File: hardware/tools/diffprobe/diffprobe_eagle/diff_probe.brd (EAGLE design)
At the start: 26.7 x 26.3 mm, 32 parts, among them U1 AD8129, X1 SMA-142-0701-801/806

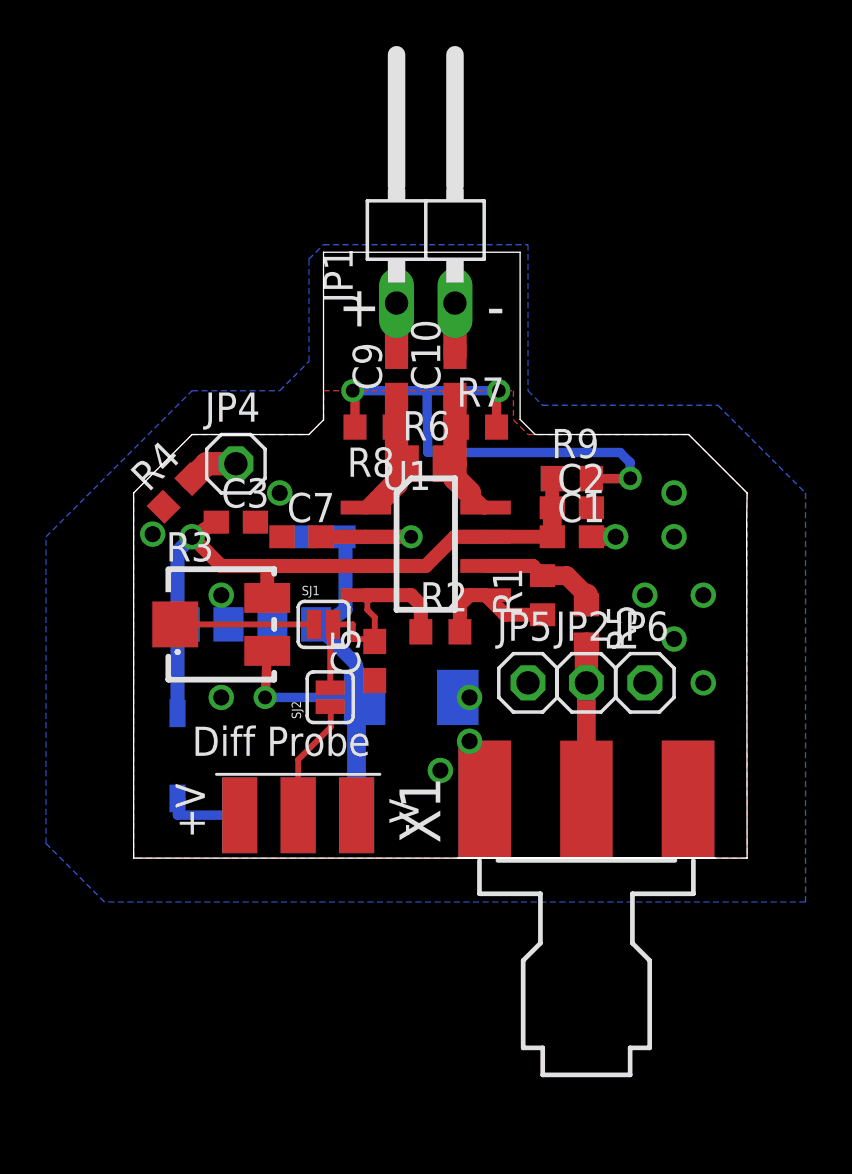
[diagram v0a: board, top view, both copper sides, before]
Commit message: HW: Update differential probe with latest design
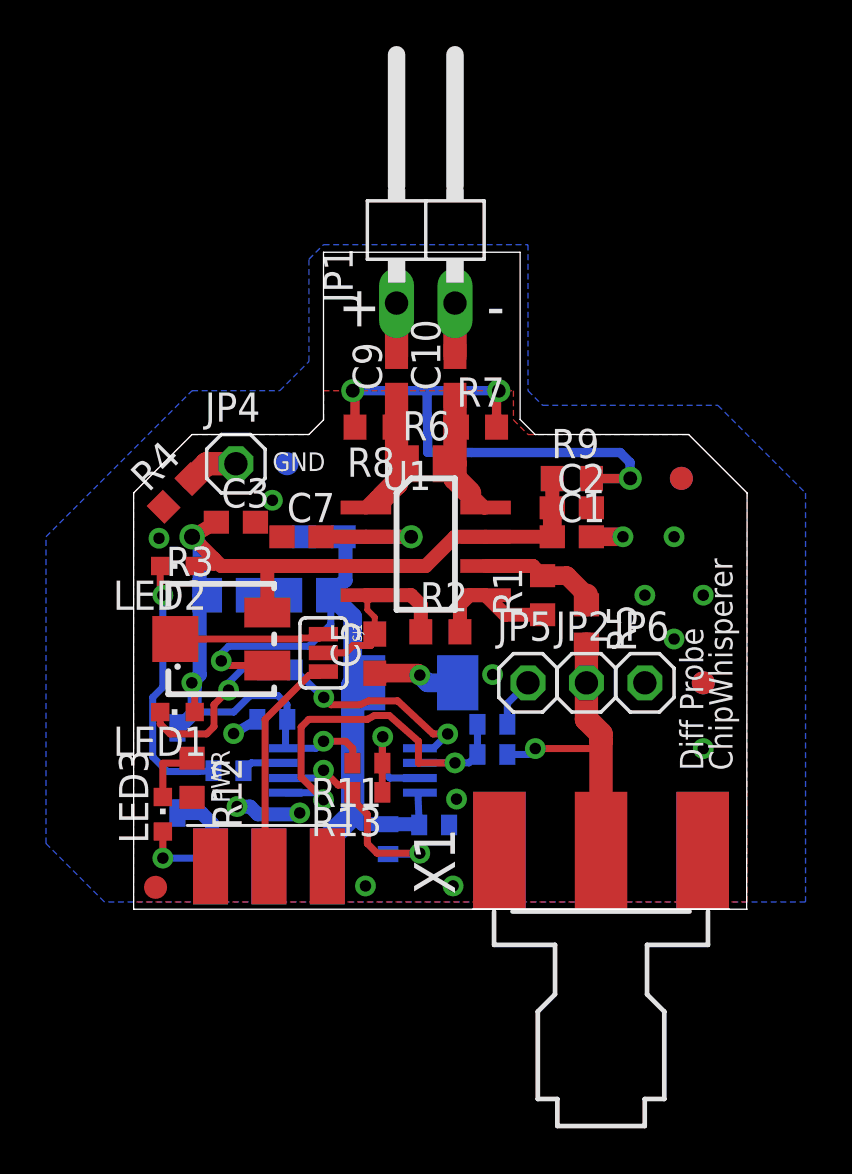
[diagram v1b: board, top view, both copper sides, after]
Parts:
- removed SJ2: SOLDERJUMPERNC, SparkFun:SJ_2S
- added C11, C12, C13: (no value), resistor:C0402
- added LED1, LED3: RIGHT, led:CHIPLED_0603
- added LED2: LEFT, led:CHIPLED_0603
- added R11, R14: 10k, 1%, rcl:R0402
- added R12: 4k7, resistor:R0603
- added R13: 510R, 1%, rcl:R0402
- added R15: 25k, rcl:R0402
- added R16, R17: (no value), rcl:R0402
- added U$1, U$2, U$3, U$4, U$5, U$6: FIDUCIAL, adafruit:FIDUCIAL_1MM
- added U2: LM2903PWR, Texas Instruments_By_element14_Batch_1:SOP65P640X120-8N
- SJ1: value SOLDERJUMPERNC -> (none); device SparkFun:SJ_2S -> SparkFun:SJ_3_PASTE1&2
- moved JP3 2.56 mm to (17.3, 13.0)
- moved X1 2.31 mm to (31.8, 11.1)
- moved C6 1.60 mm to (15.6, 24.8)
- moved C8 1.42 mm to (19.1, 24.8)
- moved SJ1 1.24 mm to (19.7, 22.3), turned to 270 degrees
- moved D1 0.64 mm to (13.3, 17.1)
- moved R3 0.64 mm to (15.2, 22.9)
- moved D2 0.63 mm to (23.5, 21.0)
- moved C5 0.32 mm to (21.9, 22.2)
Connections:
- new net N$16: R11.1, R13.1, U2.3
- new net N$17: R13.2, R14.1, U2.6
- new net N$18: R16.1, U2.1
- new net N$19: C11.2, R15.2, U2.2, U2.5
- new net N$20: LED1.C, R16.2
- new net N$21: R17.1, U2.7
- new net N$22: LED2.C, R17.2
- new net N$9: LED3.C, R12.1
- net AGND: now also C11.1, C12.2, C13.1, R12.2
- net N$1: now also LED3.A
- net N$10: now also SJ1.3; no longer SJ2.1
- net N$12: now also R15.1
- net N$2: now also C12.1, LED1.A, LED2.A, R11.2, U2.8
- net N$3: no longer SJ2.2
- net N$8: now also C13.2, R14.2, U2.4
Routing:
- net N$19: track 0.00 -> 17.6 mm, vias 0 -> 2
- net N$2: track 30.2 -> 45.5 mm, vias 1 -> 3
- net N$22: track 0.00 -> 11.4 mm, vias 0 -> 1
- net N$17: track 0.00 -> 10.6 mm, vias 0 -> 2
- net AGND: track 1.05 -> 11.4 mm, vias 14 -> 16
- net N$8: track 27.2 -> 37.3 mm
- net N$18: track 0.00 -> 9.34 mm, vias 0 -> 2
- net N$20: track 0.00 -> 7.24 mm, vias 0 -> 1
- net N$12: track 6.74 -> 13.5 mm, vias 0 -> 1
- net N$16: track 0.00 -> 6.16 mm, vias 0 -> 1
- net N$10: track 5.32 -> 10.5 mm
- net N$1: track 3.52 -> 6.94 mm, vias 0 -> 1
- net N$9: track 0.00 -> 2.83 mm
- net N$3: track 11.2 -> 8.54 mm
- net N$21: track 0.00 -> 1.97 mm
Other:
- board size 26.7 x 26.3 mm -> 26.7 x 28.6 mm
- board text added: "28OCT2014"
- board text added: "ChipWhisperer"
- board text added: "GND"
- board text added: "NPCB-DIFFPROBE-02"
- board text added: "NewAE Technology Inc"
- board text added: "PWR"
- board text added: "V+"
- board text added: "V-"
- board text removed: "+V"
- board text removed: "-V"
- board text removed: "ChipWhisperer.com"
- board text removed: "Colin O'Flynn"
- board text removed: "MAR92013"

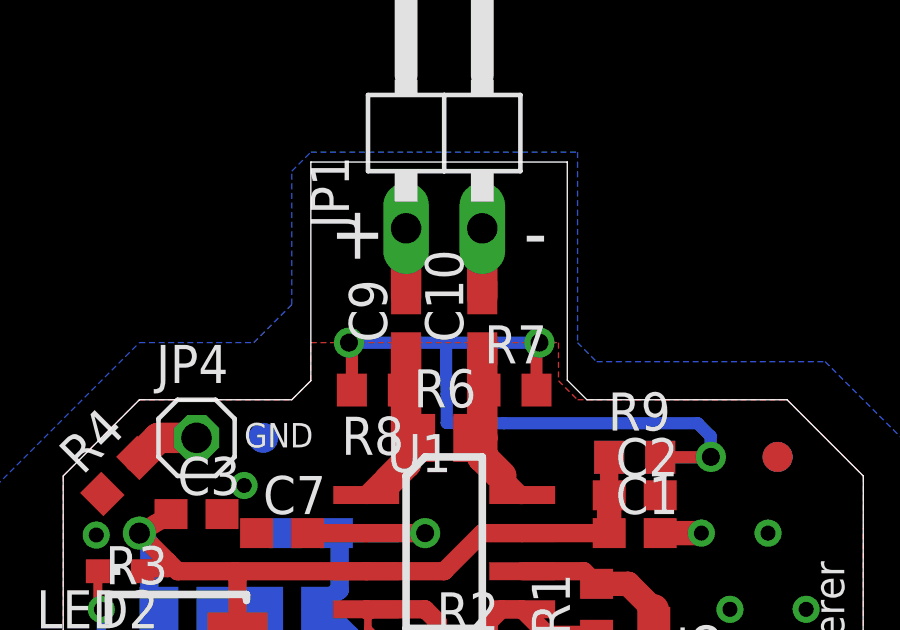
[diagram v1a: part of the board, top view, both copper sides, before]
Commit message: Update differential probe stuff
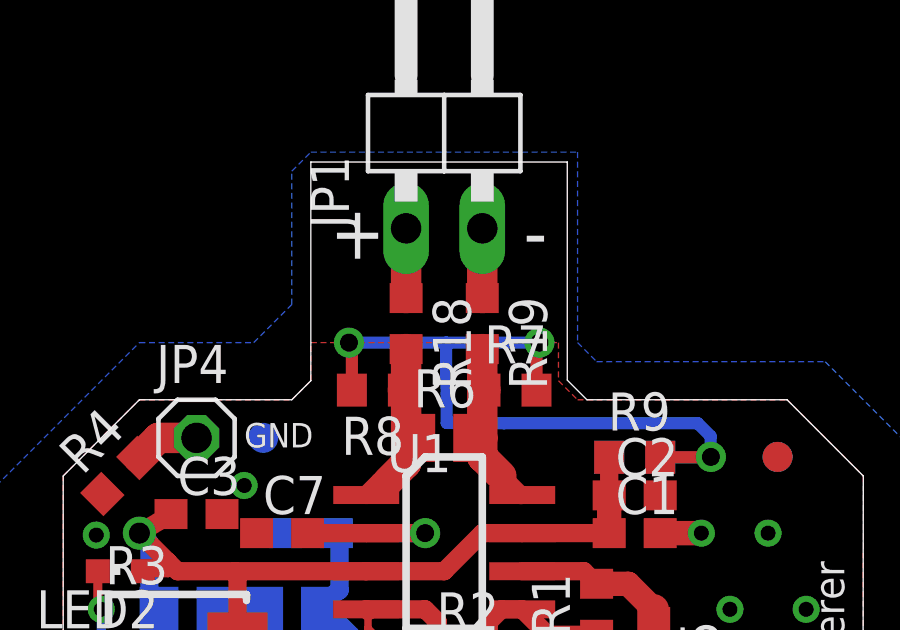
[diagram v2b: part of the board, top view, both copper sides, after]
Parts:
- removed C10, C9: 0R, rcl:C0603
- added R18, R19: 10R, resistor:R0603
- C11: value (none) -> 680pF
- C12, C13: value (none) -> 100nF
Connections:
- net N$13: now also R19.2; no longer C10.1
- net N$14: now also R19.1; no longer C10.2
- net N$6: now also R18.1; no longer C9.2
- net N$7: now also R18.2; no longer C9.1
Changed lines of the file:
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@@
 <element name="JP6" library="pinhead" package="1X01" value="" x="33.655" y="20.955"/>
 <element name="R5" library="resistor" package="R0603" value="49.9R" x="31.115" y="23.495" rot="R270"/>
-<element name="C9" library="rcl" package="C0603" value="0R" x="22.86" y="34.300159375" rot="R90"/>
-<element name="C10" library="rcl" package="C0603" value="0R" x="25.4" y="34.3001625" rot="R90"/>
 <element name="R6" library="resistor" package="M0805" value="DNM" x="24.13" y="30.48"/>
 <element name="R7" library="resistor" package="R0603" value="DNM" x="26.35758125" y="32.072578125"/>
@@
 <element name="R14" library="rcl" package="R0402" value="10k, 1%" x="22.491703125" y="14.160503125" rot="MR90"/>
 <element name="R15" library="rcl" package="R0402" value="25k" x="27.0256" y="17.840959375" rot="MR0"/>
-<element name="C11" library="resistor" package="C0402" value="" x="27.025603125" y="19.1516" rot="MR0">
+<element name="C11" library="resistor" package="C0402" value="680pF" x="27.025603125" y="19.1516" rot="MR0">
 <attribute name="SPICEPREFIX" value="C" x="27.025603125" y="19.1516" size="1.778" layer="28" rot="MR0" display="off"/>
 </element>
@@
 <element name="LED1" library="led" package="CHIPLED_0603" value="RIGHT" x="13.335" y="19.685" rot="R90"/>
 <element name="LED2" library="led" package="CHIPLED_0603" value="LEFT" x="13.335" y="26.035" rot="R90"/>
-<element name="C12" library="resistor" package="C0402" value="" x="17.457421875" y="19.3675" rot="MR0">
+<element name="C12" library="resistor" package="C0402" value="100nF" x="17.457421875" y="19.3675" rot="MR0">
 <attribute name="SPICEPREFIX" value="C" x="17.457421875" y="19.3675" size="1.778" layer="28" rot="MR0" display="off"/>
 </element>
-<element name="C13" library="resistor" package="C0402" value="" x="24.492421875" y="14.77758125" rot="MR0">
+<element name="C13" library="resistor" package="C0402" value="100nF" x="24.492421875" y="14.77758125" rot="MR0">
 <attribute name="SPICEPREFIX" value="C" x="24.492421875" y="14.77758125" size="1.778" layer="28" rot="MR0" display="off"/>
 </element>
@@
 <element name="U$5" library="adafruit" package="FIDUCIAL_1MM" value="FIDUCIAL" x="36.195" y="20.955"/>
 <element name="U$6" library="adafruit" package="FIDUCIAL_1MM" value="FIDUCIAL" x="36.195" y="20.955" rot="MR0"/>
+<element name="R18" library="resistor" package="R0603" value="10R" x="22.86" y="34.29" rot="R270"/>
+<element name="R19" library="resistor" package="R0603" value="10R" x="25.4" y="34.29" rot="R270"/>
 </elements>
 <signals>
@@
 <signal name="N$6">
 <contactref element="JP1" pad="1"/>
-<contactref element="C9" pad="2"/>
-<wire x1="22.86" y1="35.150159375" x2="22.86" y2="37.465" width="1.016" layer="1"/>
+<contactref element="R18" pad="1"/>
+<wire x1="22.86" y1="35.14" x2="22.86" y2="37.465" width="1.016" layer="1"/>
 </signal>
 <signal name="N$7">
-<contactref element="C9" pad="1"/>
 <contactref element="R6" pad="1"/>
 <contactref element="R8" pad="1"/>
 <contactref element="U1" pad="1"/>
-<wire x1="22.86" y1="33.450159375" x2="22.86" y2="31.75" width="1.016" layer="1"/>
 <wire x1="22.86" y1="31.75" x2="22.86" y2="30.48" width="1.016" layer="1"/>
 <wire x1="22.86" y1="30.48" x2="22.86" y2="29.63418125" width="1.016" layer="1"/>
@@
 <wire x1="22.25801875" y1="29.0322" x2="21.9872" y2="29.0322" width="0.6096" layer="1"/>
 <wire x1="21.9872" y1="29.0322" x2="21.53" y2="28.575" width="0.6096" layer="1"/>
+<contactref element="R18" pad="2"/>
+<wire x1="22.86" y1="33.44" x2="22.86" y2="32.18015625" width="1.016" layer="1"/>
+<wire x1="22.86" y1="32.18015625" x2="22.752421875" y2="32.072578125" width="1.016" layer="1"/>
 </signal>
 <signal name="N$13">
 <contactref element="R6" pad="2"/>
-<contactref element="C10" pad="1"/>
 <contactref element="R7" pad="1"/>
 <contactref element="U1" pad="8"/>
-<wire x1="25.4" y1="33.4501625" x2="25.4" y2="32.385" width="1.016" layer="1"/>
 <wire x1="25.4" y1="32.385" x2="25.4" y2="30.48" width="1.016" layer="1"/>
 <wire x1="25.4" y1="30.48" x2="25.4" y2="29.845" width="1.016" layer="1"/>
@@
 <wire x1="26.73" y1="28.575" x2="26.67" y2="28.575" width="0.6096" layer="1"/>
 <wire x1="26.67" y1="28.575" x2="26.035" y2="29.21" width="0.6096" layer="1"/>
+<contactref element="R19" pad="2"/>
+<wire x1="25.4" y1="33.44" x2="25.4" y2="32.180159375" width="1.016" layer="1"/>
+<wire x1="25.4" y1="32.180159375" x2="25.50758125" y2="32.072578125" width="1.016" layer="1"/>
 </signal>
 <signal name="N$14">
-<contactref element="C10" pad="2"/>
 <contactref element="JP1" pad="2"/>
-<wire x1="25.4" y1="35.1501625" x2="25.4" y2="37.465" width="1.016" layer="1"/>
+<contactref element="R19" pad="1"/>
+<wire x1="25.4" y1="35.14" x2="25.4" y2="37.465" width="1.016" layer="1"/>
 </signal>
 <signal name="N$15">

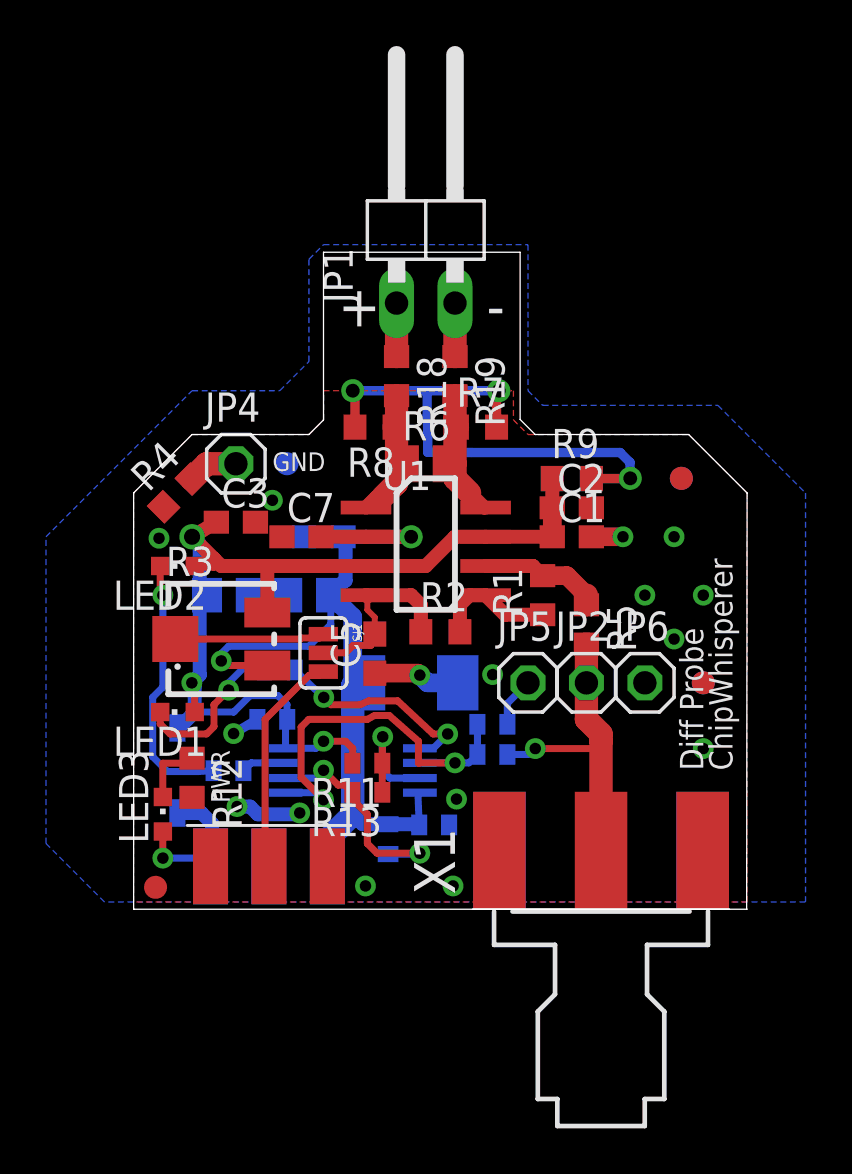
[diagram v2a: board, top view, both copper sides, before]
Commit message: HW: Update LNA + Diff probe with latest version
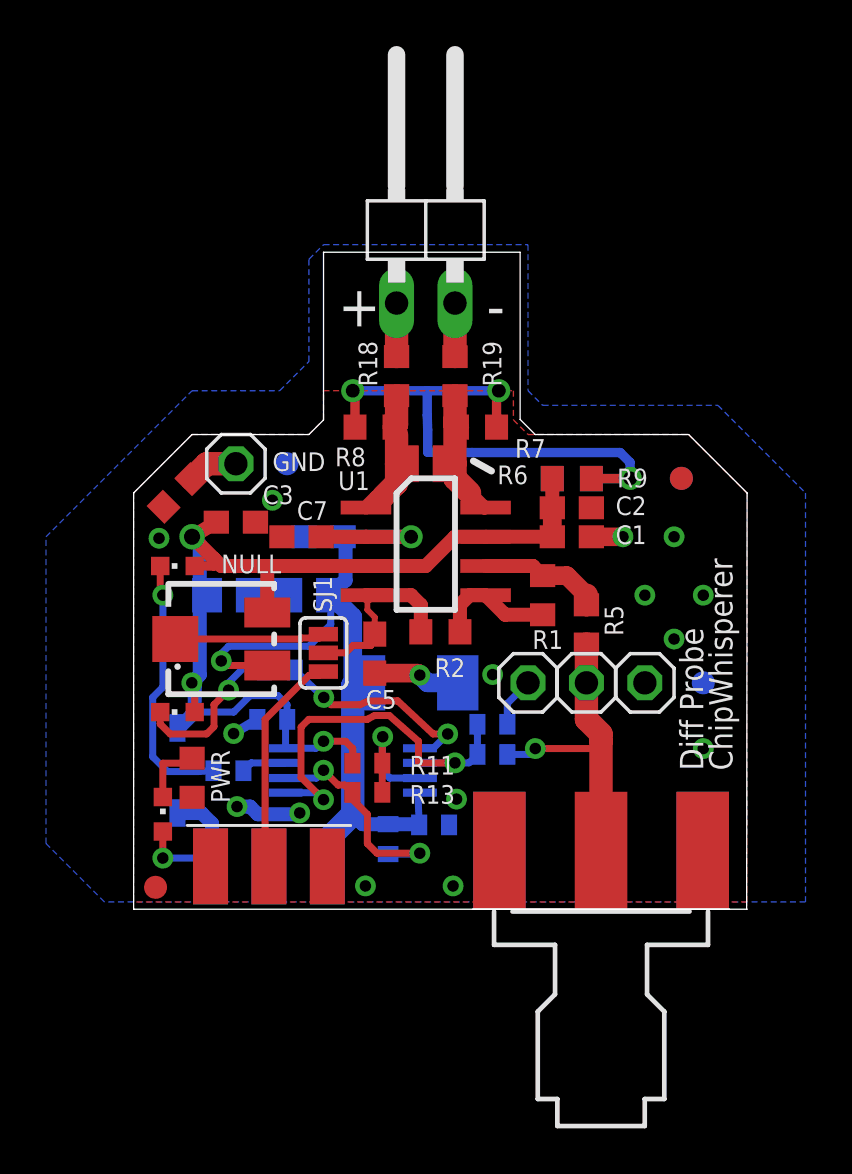
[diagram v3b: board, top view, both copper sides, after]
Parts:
- removed U$5: FIDUCIAL, adafruit:FIDUCIAL_1MM
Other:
- board text added: "NULL"

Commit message: PCBs: Add LNA/Diff-Probe updates, + firmware temp fixes
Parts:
- removed U$1, U$3: FIDUCIAL, adafruit:FIDUCIAL_1MM
- added FID2, FID5: FIDUCIAL, adafruit:FIDUCIAL_1MM
- R13: value 510R, 1% -> 1k, 1%
- renumbered U$2 to FID4, U$4 to FID1, U$6 to FID6
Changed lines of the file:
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@@
 <?xml version="1.0" encoding="utf-8"?>
 <!DOCTYPE eagle SYSTEM "eagle.dtd">
-<eagle version="7.1.0">
+<eagle version="7.2.0">
 <drawing>
 <settings>
@@
 <grid distance="0.3175" unitdist="mm" unit="mm" style="lines" multiple="1" display="no" altdistance="0.05" altunitdist="mm" altunit="mm"/>
 <layers>
-<layer number="1" name="Top" color="4" fill="1" visible="no" active="yes"/>
+<layer number="1" name="Top" color="4" fill="1" visible="yes" active="yes"/>
 <layer number="2" name="Route2" color="1" fill="3" visible="no" active="no"/>
 <layer number="3" name="Route3" color="4" fill="3" visible="no" active="no"/>
@@
 <layer number="19" name="Unrouted" color="6" fill="1" visible="yes" active="yes"/>
 <layer number="20" name="Dimension" color="15" fill="1" visible="yes" active="yes"/>
-<layer number="21" name="tPlace" color="7" fill="1" visible="no" active="yes"/>
+<layer number="21" name="tPlace" color="7" fill="1" visible="yes" active="yes"/>
 <layer number="22" name="bPlace" color="7" fill="1" visible="yes" active="yes"/>
-<layer number="23" name="tOrigins" color="15" fill="1" visible="no" active="yes"/>
+<layer number="23" name="tOrigins" color="15" fill="1" visible="yes" active="yes"/>
 <layer number="24" name="bOrigins" color="15" fill="1" visible="no" active="yes"/>
 <layer number="25" name="tNames" color="7" fill="1" visible="no" active="yes"/>
@@
 <attribute name="VALUE" x="22.225" y="19.3675" size="1.27" layer="27" rot="R180"/>
 </element>
-<element name="R13" library="rcl" package="R0402" value="510R, 1%" x="21.59" y="16.1925" smashed="yes" rot="R180">
+<element name="R13" library="rcl" package="R0402" value="1k, 1%" x="21.59" y="16.1925" smashed="yes" rot="R180">
 <attribute name="NAME" x="25.4" y="16.51" size="0.8128" layer="25" font="vector" ratio="16" rot="R180"/>
 <attribute name="VALUE" x="22.225" y="18.0975" size="1.27" layer="27" rot="R180"/>
@@
 <attribute name="VALUE" x="11.938" y="17.7165" size="1.27" layer="27" rot="R270"/>
 </element>
-<element name="U$1" library="adafruit" package="FIDUCIAL_1MM" value="FIDUCIAL" x="35.2425" y="29.845" rot="MR0"/>
-<element name="U$2" library="adafruit" package="FIDUCIAL_1MM" value="FIDUCIAL" x="18.0975" y="30.48" smashed="yes" rot="MR0"/>
-<element name="U$3" library="adafruit" package="FIDUCIAL_1MM" value="FIDUCIAL" x="35.2425" y="29.845"/>
-<element name="U$4" library="adafruit" package="FIDUCIAL_1MM" value="FIDUCIAL" x="12.3825" y="12.065"/>
-<element name="U$6" library="adafruit" package="FIDUCIAL_1MM" value="FIDUCIAL" x="36.195" y="20.955" rot="MR0"/>
+<element name="FID5" library="adafruit" package="FIDUCIAL_1MM" value="FIDUCIAL" x="35.2425" y="29.845" rot="MR0"/>
+<element name="FID4" library="adafruit" package="FIDUCIAL_1MM" value="FIDUCIAL" x="18.0975" y="30.48" smashed="yes" rot="MR0"/>
+<element name="FID2" library="adafruit" package="FIDUCIAL_1MM" value="FIDUCIAL" x="35.2425" y="29.845"/>
+<element name="FID1" library="adafruit" package="FIDUCIAL_1MM" value="FIDUCIAL" x="12.3825" y="12.065"/>
+<element name="FID6" library="adafruit" package="FIDUCIAL_1MM" value="FIDUCIAL" x="36.195" y="20.955" rot="MR0"/>
 <element name="R18" library="resistor" package="R0603" value="10R" x="22.86" y="34.29" smashed="yes" rot="R270">
 <attribute name="NAME" x="21.209" y="35.814" size="0.8128" layer="25" font="vector" ratio="16" rot="R270"/>
